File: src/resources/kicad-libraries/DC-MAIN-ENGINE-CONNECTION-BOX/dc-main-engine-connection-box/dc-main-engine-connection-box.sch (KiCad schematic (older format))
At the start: 12 parts, among them K1 MAIN ENGINE START, K2 SHAFT LUBE PUMP

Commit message: .
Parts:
- U?: symbol trollvalve:POLOLU_TIC_T500 -> dc-main-engine-connection-box-rescue:POLOLU_TIC_T500-trollvalve
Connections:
- net labels added: SOLENOID_+24VDC, SOLENOID_GND
- net labels removed: +24VDC_SOLENOID, GND_SOLENOID
- wire segments 108 -> 111
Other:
- note added: "4"
- note added: "5"
- note added: "7"
- note added: "HELM PANEL LOOM (MULTICORE)"
- note added: "TROLL LOOM (MULTICORE)"
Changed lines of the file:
@@
 U 1 1 5E200D1B
 P 2250 5600
-F 0 "J?" H 2168 6317 50  0000 C CNN
-F 1 "Screw_Terminal_01x12" H 2168 6226 50  0000 C CNN
+F 0 "J?" H 2168 6317 50  0001 C CNN
+F 1 "Screw_Terminal_01x12" H 2168 6226 50  0001 C CNN
 F 2 "" H 2250 5600 50  0001 C CNN
 F 3 "~" H 2250 5600 50  0001 C CNN
@@
 TROLL_POSITION
 Text Notes 2150 5000 2    40   ~ 0
-ENGINE LOOM
+HELM PANEL LOOM (MULTICORE)
 Wire Wire Line
 	4100 1600 4000 1600
@@
 	5000 1700 5000 2000
 Wire Wire Line
-	5000 2000 9300 2000
-Wire Wire Line
 	2000 4000 6800 4000
 Wire Wire Line
 	6800 4000 6800 1800
-Wire Wire Line
-	6800 1800 9250 1800
-Wire Wire Line
-	6400 1700 9250 1700
 Connection ~ 2000 4000
 Wire Wire Line
 	2000 4000 2000 4100
 Wire Wire Line
-	9300 2100 6900 2100
-Wire Wire Line
-	6900 5600 2450 5600
+	7050 5600 2450 5600
 Connection ~ 2450 5600
 Wire Wire Line
-	7000 5700 7000 2200
-Wire Wire Line
-	7000 2200 9300 2200
-Wire Wire Line
-	2450 5700 7000 5700
+	7150 5700 7150 2200
+Wire Wire Line
+	2450 5700 7150 5700
 Connection ~ 2450 5700
 Wire Wire Line
-	9300 2300 7100 2300
-Wire Wire Line
-	7100 5800 2450 5800
+	7250 5800 2450 5800
 Connection ~ 2450 5800
 Wire Wire Line
 	5400 1200 5400 5400
 Wire Wire Line
-	6900 2100 6900 5600
-Wire Wire Line
-	7100 2300 7100 5800
+	7050 2100 7050 5600
+Wire Wire Line
+	7250 2300 7250 5800
 Wire Wire Line
 	3900 1200 3900 5200
 Wire Wire Line
-	2450 5900 7200 5900
-Wire Wire Line
-	7200 5900 7200 2400
-Wire Wire Line
-	7200 2400 9300 2400
+	2450 5900 7350 5900
+Wire Wire Line
+	7350 5900 7350 2400
 Connection ~ 2450 5900
 Wire Wire Line
@@
 Connection ~ 2000 4100
 Wire Wire Line
-	2450 5500 7300 5500
+	2450 5500 7450 5500
 Connection ~ 2450 5500
 Connection ~ 2450 6200
 $Comp
-L trollvalve:POLOLU_TIC_T500 U?
+L dc-main-engine-connection-box-rescue:POLOLU_TIC_T500-trollvalve U?
 U 1 1 5E31D2A1
 P 8500 4200
@@
 	2000 3800 8000 3800
 Wire Wire Line
-	8000 4300 7400 4300
-Wire Wire Line
-	7400 4300 7400 5400
-Wire Wire Line
-	8000 4400 7500 4400
-Wire Wire Line
-	7500 4400 7500 5300
-Wire Wire Line
-	7600 4500 7600 5200
-Wire Wire Line
-	7600 4500 8000 4500
-Wire Wire Line
-	8000 4600 7700 4600
-Wire Wire Line
-	7700 4600 7700 5100
-Wire Wire Line
-	8000 3700 7300 3700
-Wire Wire Line
-	7300 3700 7300 5500
-Connection ~ 7300 5500
+	8000 4300 7550 4300
+Wire Wire Line
+	7550 4300 7550 5400
+Wire Wire Line
+	8000 4400 7650 4400
+Wire Wire Line
+	7650 4400 7650 5300
+Wire Wire Line
+	7750 4500 7750 5200
+Wire Wire Line
+	7750 4500 8000 4500
+Wire Wire Line
+	8000 4600 7850 4600
+Wire Wire Line
+	7850 4600 7850 5100
+Wire Wire Line
+	8000 3700 7450 3700
+Wire Wire Line
+	7450 3700 7450 4900
 Wire Wire Line
 	9200 6200 9200 4000
@@
 	9100 3900 9400 3900
 Wire Wire Line
-	9400 3900 9400 4900
-Wire Wire Line
-	9400 4900 10000 4900
-Wire Wire Line
-	7700 5100 10000 5100
-Wire Wire Line
-	7600 5200 10000 5200
-Wire Wire Line
-	7500 5300 10000 5300
-Wire Wire Line
-	7400 5400 10000 5400
-Wire Wire Line
-	7300 5500 10000 5500
+	9400 3900 9400 4600
+Wire Wire Line
+	9400 4600 10000 4600
+Wire Wire Line
+	7850 5100 10000 5100
+Wire Wire Line
+	7750 5200 10000 5200
+Wire Wire Line
+	7650 5300 10000 5300
+Wire Wire Line
+	7550 5400 10000 5400
 Wire Wire Line
 	2450 6200 9200 6200
 Wire Wire Line
 	2000 4300 2550 4300
-Connection ~ 2000 4300
-Wire Wire Line
-	2000 4300 2000 4750
 Wire Wire Line
 	2550 4300 2550 6000
@@
 	2000 4200 2000 4300
 Text GLabel 10000 4800 2    50   Output ~ 0
-GND_SOLENOID
-Text GLabel 10000 4900 2    50   Input ~ 0
+SOLENOID_GND
+Text GLabel 10000 4600 2    50   Input ~ 0
 LIMIT_SWITCH
-Text GLabel 10000 5500 2    50   Output ~ 0
-+24VDC_SOLENOID
+Text GLabel 10000 4900 2    50   Output ~ 0
+SOLENOID_+24VDC
 Text GLabel 10000 5100 2    50   Output ~ 0
 MOTOR_A
@@
 Text GLabel 10000 5400 2    50   Output ~ 0
 MOTOR_B
+Wire Wire Line
+	10000 4900 7450 4900
+Connection ~ 7450 4900
+Wire Wire Line
+	7450 4900 7450 5500
+Wire Notes Line
+	9600 4500 9750 4500
+Wire Notes Line
+	9750 4500 9750 5500
+Wire Notes Line
+	9750 5500 9600 5500
+Wire Notes Line
+	9600 5500 9600 4500
+Text Notes 9600 4500 0    50   ~ 0
+TROLL LOOM (MULTICORE)
+Text Notes 9600 4900 0    50   ~ 0
+1
+Text Notes 9600 4800 0    50   ~ 0
+2
+Text Notes 9600 4600 0    50   ~ 0
+3
+Text Notes 9600 5100 0    50   ~ 0
+4
+Text Notes 9600 5200 0    50   ~ 0
+5
+Text Notes 9600 5300 0    50   ~ 0
+6
+Text Notes 9600 5400 0    50   ~ 0
+7
+Wire Wire Line
+	7350 2400 10000 2400
+Wire Wire Line
+	7250 2300 10000 2300
+Wire Wire Line
+	7150 2200 10000 2200
+Wire Wire Line
+	7050 2100 10000 2100
+Wire Wire Line
+	5000 2000 10000 2000
+Wire Wire Line
+	6800 1800 10000 1800
+Wire Wire Line
+	6400 1700 10000 1700
+Wire Notes Line
+	9600 2500 9750 2500
+Wire Notes Line
+	9750 2500 9750 1600
+Wire Notes Line
+	9750 1600 9600 1600
+Wire Notes Line
+	9600 1600 9600 2500
+Text Notes 9600 1600 0    50   ~ 0
+ENGINE LOOM
+Wire Wire Line
+	2450 5300 6950 5300
+Wire Wire Line
+	6950 5300 6950 1900
+Wire Wire Line
+	6950 1900 10000 1900
+Connection ~ 2450 5300
 $EndSCHEMATC

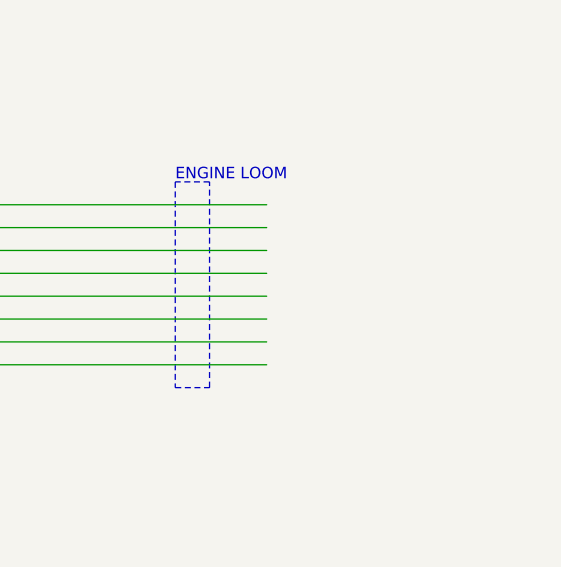
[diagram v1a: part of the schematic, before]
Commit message: .
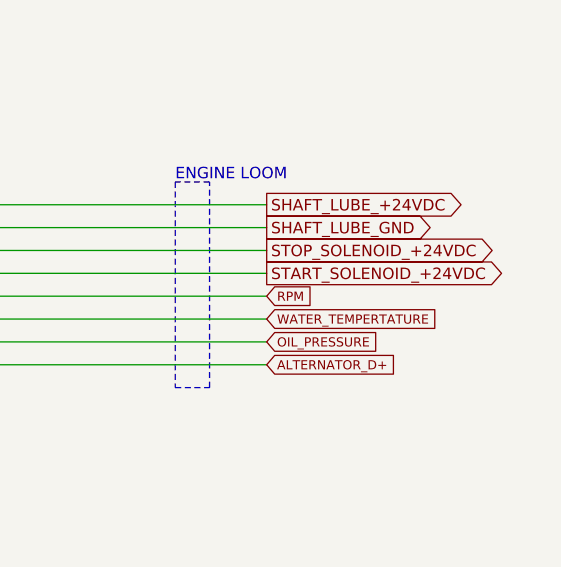
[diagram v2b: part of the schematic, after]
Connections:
- net labels added: SHAFT_LUBE_+24VDC, SHAFT_LUBE_GND, START_SOLENOID_+24VDC, STOP_SOLENOID_+24VDC
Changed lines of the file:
@@
 Rev ""
 Comp ""
-Comment1 ""
+Comment1 "TROLL_ON and TROLL_POSITION fused at helm."
 Comment2 ""
 Comment3 ""
@@
 	6950 1900 10000 1900
 Connection ~ 2450 5300
+Text GLabel 10000 1700 2    50   Output ~ 0
+SHAFT_LUBE_+24VDC
+Text GLabel 10000 1800 2    50   Output ~ 0
+SHAFT_LUBE_GND
+Text GLabel 10000 1900 2    50   Output ~ 0
+STOP_SOLENOID_+24VDC
+Text GLabel 10000 2000 2    50   Output ~ 0
+START_SOLENOID_+24VDC
+Text GLabel 10000 2100 2    40   Input ~ 0
+RPM
+Text GLabel 10000 2200 2    40   Input ~ 0
+WATER_TEMPERTATURE
+Text GLabel 10000 2300 2    40   Input ~ 0
+OIL_PRESSURE
+Text GLabel 10000 2400 2    40   Input ~ 0
+ALTERNATOR_D+
 $EndSCHEMATC

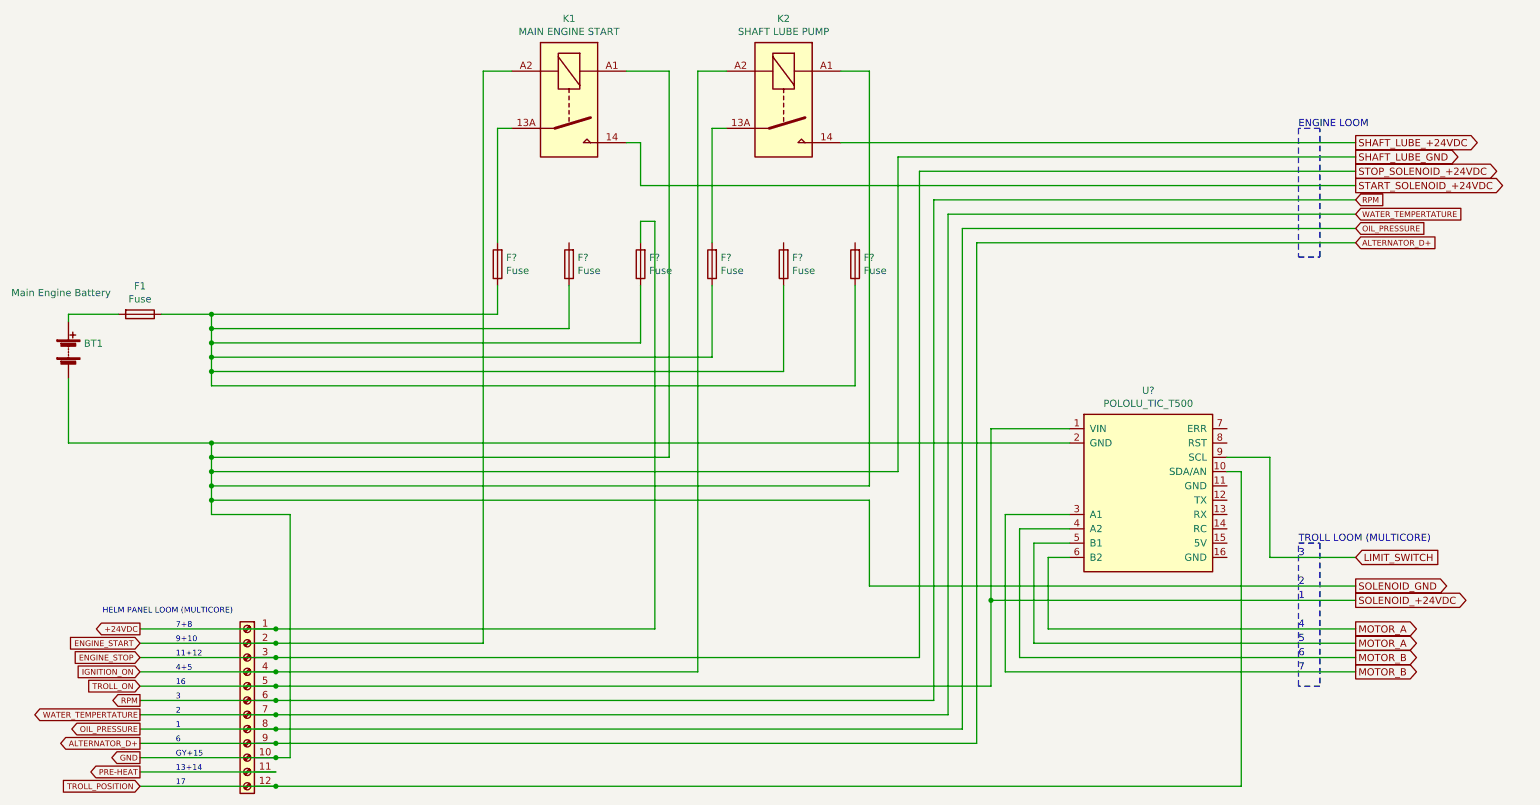
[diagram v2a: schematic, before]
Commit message: .
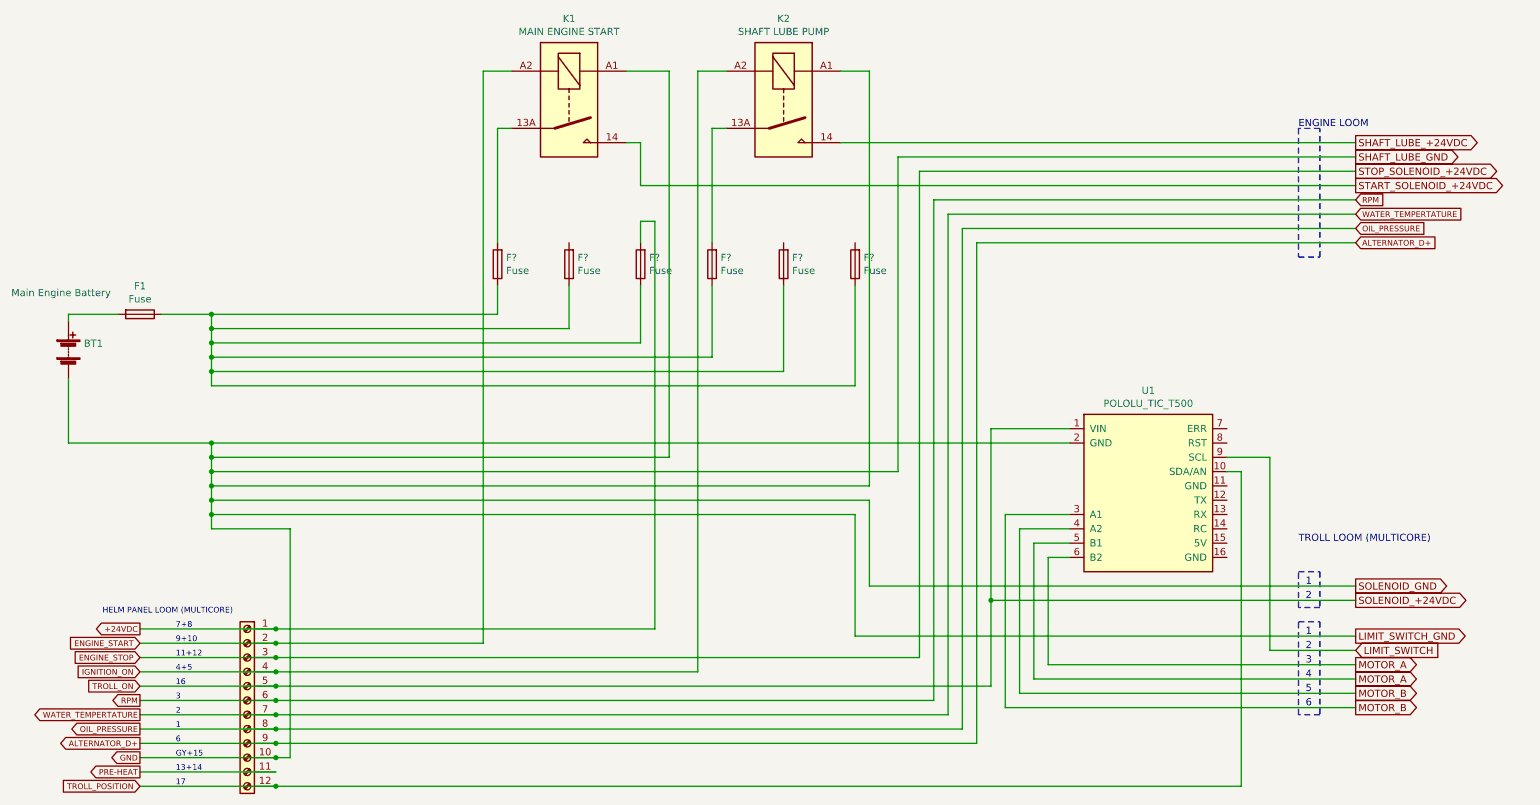
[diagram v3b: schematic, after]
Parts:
- gave numbers to parts that had none: 1
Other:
- note removed: "7"
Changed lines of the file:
@@
 Connection ~ 2450 6200
 $Comp
-L dc-main-engine-connection-box-rescue:POLOLU_TIC_T500-trollvalve U?
+L dc-main-engine-connection-box-rescue:POLOLU_TIC_T500-trollvalve U1
 U 1 1 5E31D2A1
 P 8500 4200
-F 0 "U?" H 8550 4967 50  0000 C CNN
+F 0 "U1" H 8550 4967 50  0000 C CNN
 F 1 "POLOLU_TIC_T500" H 8550 4876 50  0000 C CNN
 F 2 "Pololu_TIC_T500" H 8700 4950 50  0001 L CNN
@@
 	8000 4300 7550 4300
 Wire Wire Line
-	7550 4300 7550 5400
+	7550 4300 7550 5650
 Wire Wire Line
 	8000 4400 7650 4400
 Wire Wire Line
-	7650 4400 7650 5300
+	7650 4400 7650 5550
 Wire Wire Line
-	7750 4500 7750 5200
+	7750 4500 7750 5450
 Wire Wire Line
 	7750 4500 8000 4500
@@
 	8000 4600 7850 4600
 Wire Wire Line
-	7850 4600 7850 5100
+	7850 4600 7850 5350
 Wire Wire Line
 	8000 3700 7450 3700
@@
 	9100 3900 9400 3900
 Wire Wire Line
-	9400 3900 9400 4600
+	7850 5350 10000 5350
 Wire Wire Line
-	9400 4600 10000 4600
+	7750 5450 10000 5450
 Wire Wire Line
-	7850 5100 10000 5100
+	7650 5550 10000 5550
 Wire Wire Line
-	7750 5200 10000 5200
-Wire Wire Line
-	7650 5300 10000 5300
-Wire Wire Line
-	7550 5400 10000 5400
+	7550 5650 10000 5650
 Wire Wire Line
 	2450 6200 9200 6200
-Wire Wire Line
-	2000 4300 2550 4300
-Wire Wire Line
-	2550 4300 2550 6000
 Wire Wire Line
 	2000 4100 2000 4200
@@
 Wire Wire Line
 	6600 4200 6600 4800
-Wire Wire Line
-	6600 4800 10000 4800
 Connection ~ 2000 4200
 Wire Wire Line
 	2000 4200 2000 4300
-Text GLabel 10000 4800 2    50   Output ~ 0
-SOLENOID_GND
-Text GLabel 10000 4600 2    50   Input ~ 0
+Text GLabel 10000 5250 2    50   Input ~ 0
 LIMIT_SWITCH
 Text GLabel 10000 4900 2    50   Output ~ 0
 SOLENOID_+24VDC
-Text GLabel 10000 5100 2    50   Output ~ 0
+Text GLabel 10000 5350 2    50   Output ~ 0
 MOTOR_A
-Text GLabel 10000 5200 2    50   Output ~ 0
+Text GLabel 10000 5450 2    50   Output ~ 0
 MOTOR_A
-Text GLabel 10000 5300 2    50   Output ~ 0
+Text GLabel 10000 5550 2    50   Output ~ 0
 MOTOR_B
-Text GLabel 10000 5400 2    50   Output ~ 0
+Text GLabel 10000 5650 2    50   Output ~ 0
 MOTOR_B
 Wire Wire Line
@@
 	7450 4900 7450 5500
 Wire Notes Line
-	9600 4500 9750 4500
+	9600 4700 9750 4700
 Wire Notes Line
-	9750 4500 9750 5500
+	9750 4700 9750 4950
 Wire Notes Line
-	9750 5500 9600 5500
+	9750 4950 9600 4950
 Wire Notes Line
-	9600 5500 9600 4500
+	9600 4950 9600 4700
 Text Notes 9600 4500 0    50   ~ 0
 TROLL LOOM (MULTICORE)
-Text Notes 9600 4900 0    50   ~ 0
+Text Notes 9650 4800 0    50   ~ 0
 1
-Text Notes 9600 4800 0    50   ~ 0
+Text Notes 9650 4900 0    50   ~ 0
 2
-Text Notes 9600 4600 0    50   ~ 0
+Text Notes 9650 5350 0    50   ~ 0
 3
-Text Notes 9600 5100 0    50   ~ 0
+Text Notes 9650 5450 0    50   ~ 0
 4
-Text Notes 9600 5200 0    50   ~ 0
+Text Notes 9650 5550 0    50   ~ 0
 5
-Text Notes 9600 5300 0    50   ~ 0
+Text Notes 9650 5650 0    50   ~ 0
 6
-Text Notes 9600 5400 0    50   ~ 0
-7
 Wire Wire Line
 	7350 2400 10000 2400
@@
 Text GLabel 10000 2400 2    40   Input ~ 0
 ALTERNATOR_D+
+Wire Wire Line
+	9400 5250 10000 5250
+Wire Wire Line
+	9400 3900 9400 5250
+Wire Wire Line
+	6600 4800 10000 4800
+Text GLabel 10000 4800 2    50   Output ~ 0
+SOLENOID_GND
+Text GLabel 10000 5150 2    50   Output ~ 0
+LIMIT_SWITCH_GND
+Wire Wire Line
+	6500 5150 10000 5150
+Wire Wire Line
+	6500 4300 6500 5150
+Text Notes 9650 5250 0    50   ~ 0
+2
+Text Notes 9650 5150 0    50   ~ 0
+1
+Wire Notes Line
+	9600 5050 9750 5050
+Wire Notes Line
+	9750 5050 9750 5700
+Wire Notes Line
+	9750 5700 9600 5700
+Wire Notes Line
+	9600 5700 9600 5050
+Wire Wire Line
+	2000 4300 2000 4400
+Wire Wire Line
+	2000 4400 2550 4400
+Connection ~ 2000 4300
+Wire Wire Line
+	2550 4400 2550 6000
+Wire Wire Line
+	2000 4300 6500 4300
 $EndSCHEMATC
